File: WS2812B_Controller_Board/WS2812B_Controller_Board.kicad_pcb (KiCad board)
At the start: 2 copper layers, 43.2 x 46 mm, 13 parts, among them J1 USB_B_Micro, J2 Conn_01x03, SW1 SW_SPDT, U1 ATtiny85-20PU

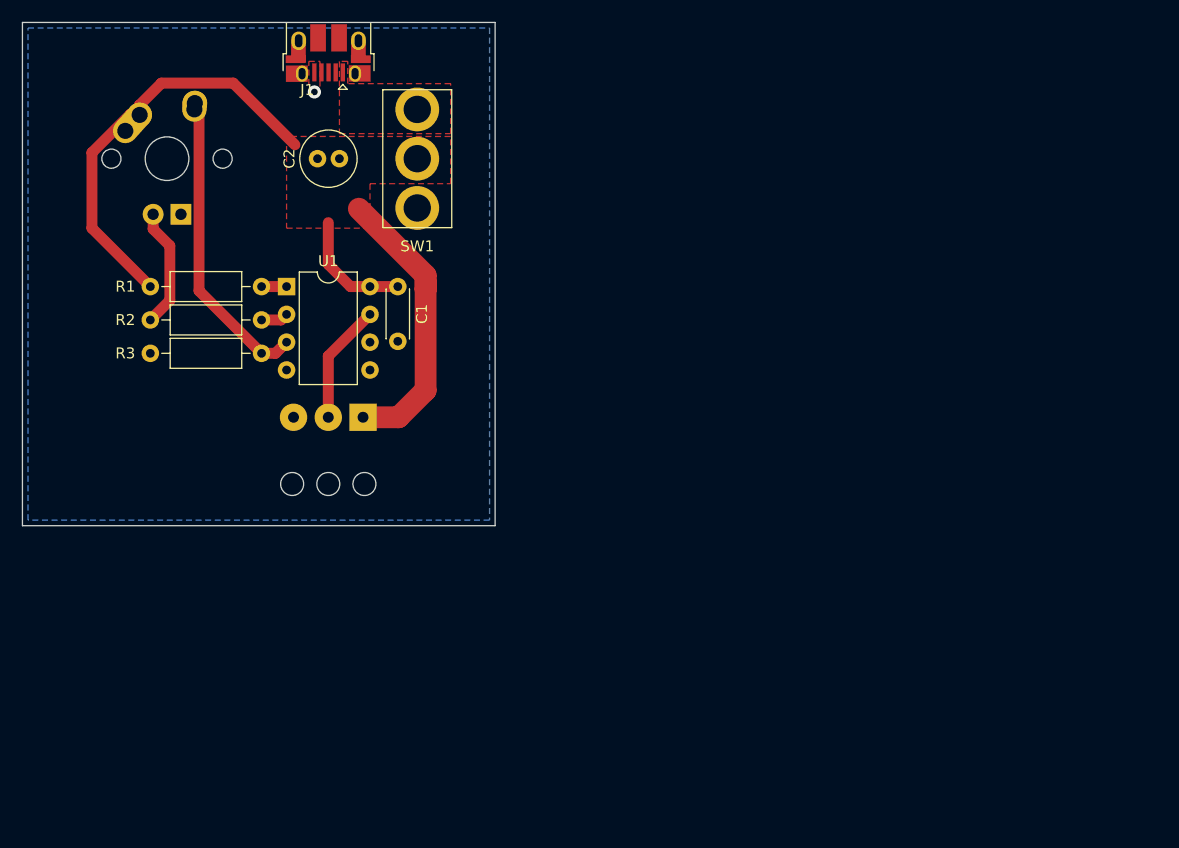
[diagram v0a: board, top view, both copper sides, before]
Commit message: Finish circuit board design
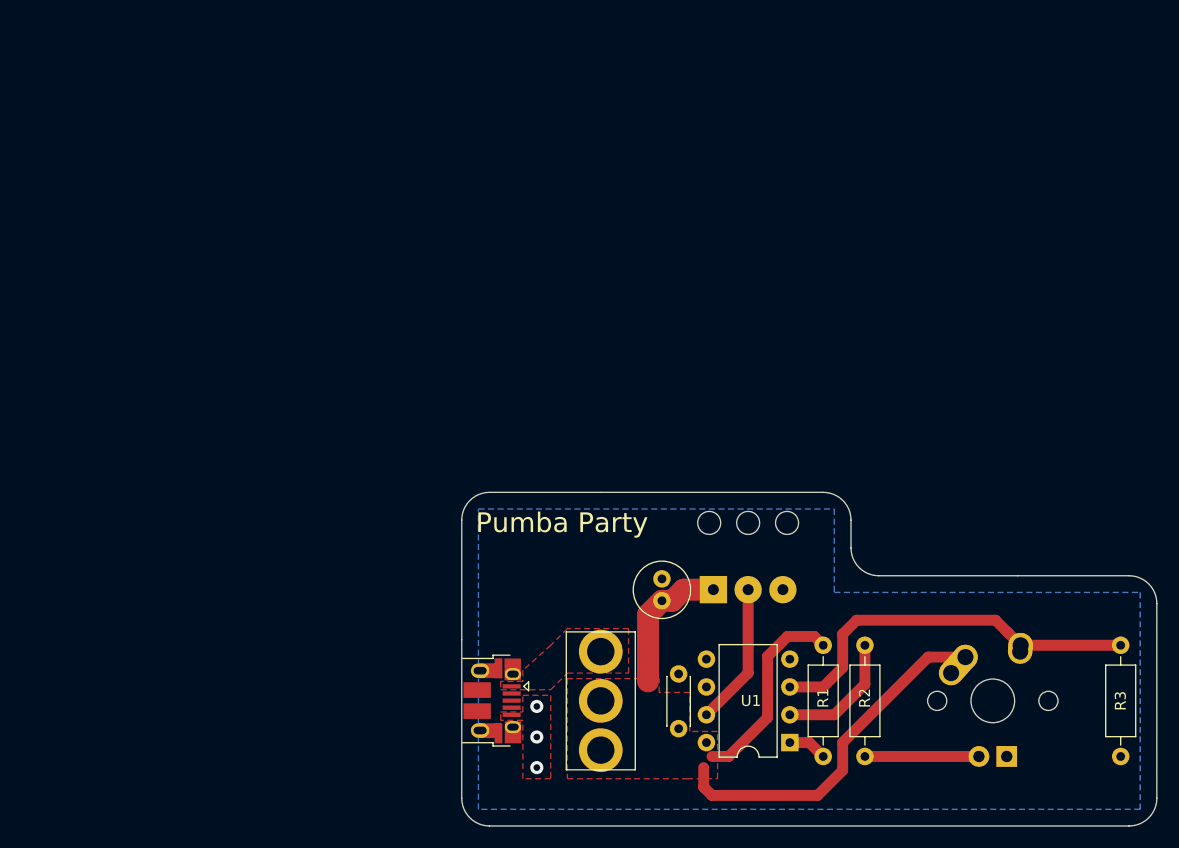
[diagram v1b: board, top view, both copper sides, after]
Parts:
- removed the REF** at (102.4, 75.4)
- removed the REF** at (99.1, 75.4)
- removed the REF** at (95.8, 75.4)
- added REF**: MountingHole_2.1mm, MountingHole:MountingHole_2.1mm, F.Cu at (133.9, 79.0)
- added REF**: MountingHole_2.1mm, MountingHole:MountingHole_2.1mm, F.Cu at (137.4, 79.0)
- added REF**: MountingHole_2.1mm, MountingHole:MountingHole_2.1mm, F.Cu at (141.0, 79.0)
- moved MX1 90.2 mm to (159.8, 95.2)
- moved R3 82.9 mm to (171.4, 90.2), turned to 270 degrees
- moved R1 69.7 mm to (144.3, 90.2), turned to 270 degrees
- moved R2 62.6 mm to (148.1, 90.2), turned to 270 degrees
- moved U1 62.0 mm to (141.2, 99.1), turned to 180 degrees
- moved J1 61.0 mm to (114.0, 95.2), turned to 270 degrees
- moved SW1 52.3 mm to (124.0, 95.2)
- moved C2 50.0 mm to (129.5, 86.1), turned to 90 degrees
- moved C1 47.8 mm to (131.1, 97.8), turned to 90 degrees
- moved J2 35.7 mm to (134.2, 85.1), turned to 0 degrees
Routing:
- net +5V: track 76.0 -> 64.0 mm
- net Net-(R2-Pad1): track 2.50 -> 11.6 mm
- net Net-(MX1-Pad2): track 27.8 -> 35.5 mm
- net Net-(J2-Pad2): track 11.0 -> 13.0 mm
- net Net-(R1-Pad2): track 2.29 -> 3.57 mm
- net Net-(MX1-Pad3): track 11.0 -> 10.4 mm
- net GND: vias 1 -> 3
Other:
- board size 43.2 x 46 mm -> 63.5 x 30.5 mm
- board text added: "Pumba Party"
- board text added: "Pumba Party Controller v1 - Designed by Aaron Lucas"
